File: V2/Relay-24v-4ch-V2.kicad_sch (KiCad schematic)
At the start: 25 parts, among them J1 DB141V-2.54-5P, J3 DB142V-5.08-2P, K1 SRD-24VDC-SL-A, K2 SRD-24VDC-SL-A, K3 SRD-24VDC-SL-A, K4 SRD-24VDC-SL-A

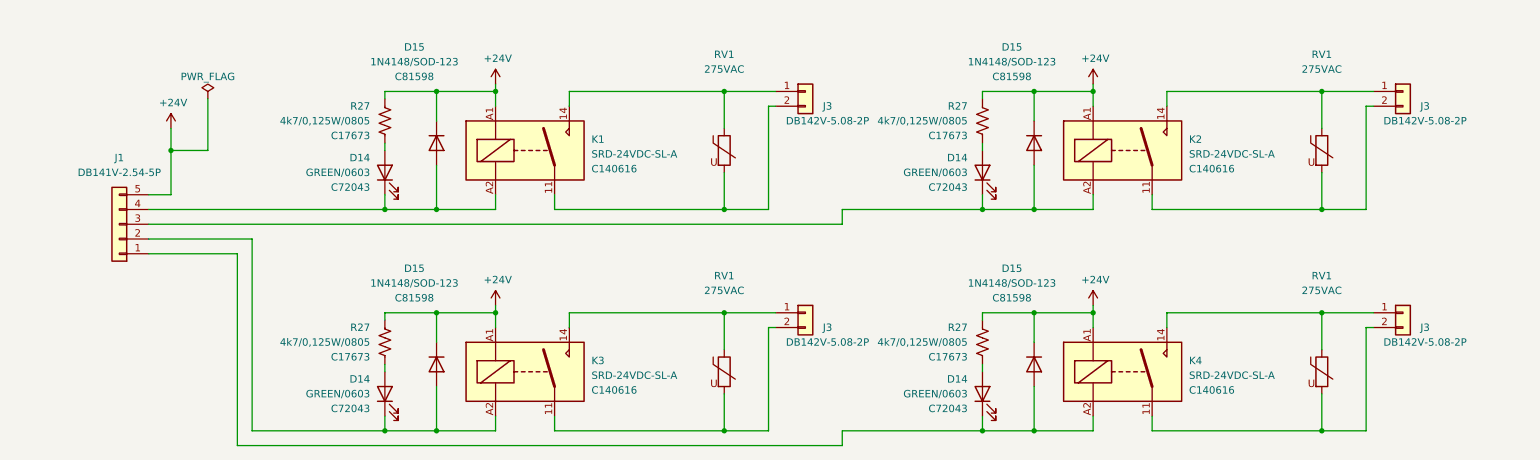
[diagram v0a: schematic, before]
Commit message: Redone everything
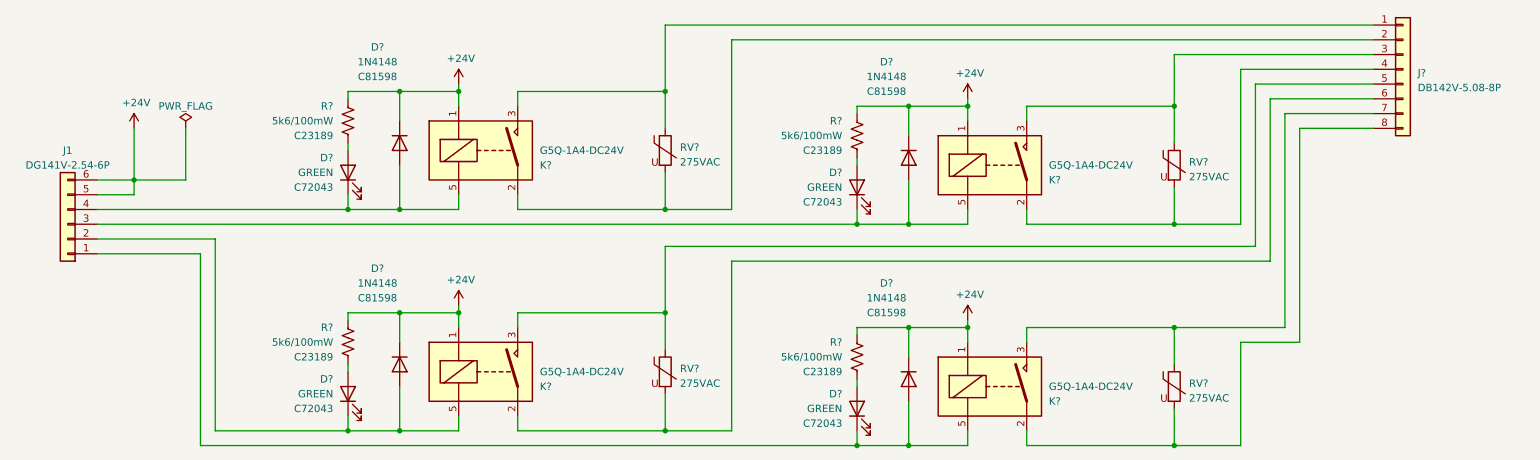
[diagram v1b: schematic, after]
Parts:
- removed J3 (x3): DB142V-5.08-2P, Tales:TerminalBlock_Dibo_DB142V-5.08-2P_1x02_P5.08mm_Vertical, symbol Connector_Generic:Conn_01x02
- removed K1, K2, K3, K4: SRD-24VDC-SL-A, Tales:Relay_SPST_Songle_SRD_FormA, symbol Tales:Songle_SRD
- added K? (x4): G5Q-1A4-DC24V, Tales:Relay_SPST_Omron-G5Q-1A, symbol Tales:G5Q-1A
- D? (x4): renamed from D14; value GREEN/0603 -> GREEN; Case 0603 -> (none); Package (none) -> 0603/1608
- D? (x4): renamed from D15; value 1N4148/SOD-123 -> 1N4148; Case SOD-123 -> (none); Package (none) -> SOD-123
- J1: value DB141V-2.54-5P -> DG141V-2.54-6P; footprint Tales:TerminalBlock_Dibo_DB141V-2.54-5P_1x05_P2.54mm_Vertical -> Tales:TerminalBlock_Dibo_DB141V-2.54-6P_1x06_P2.54mm_Vertical; symbol Connector_Generic:Conn_01x05 -> Connector_Generic:Conn_01x06; Mfr Dibo -> DIBO
- J?: renamed from J3; value DB142V-5.08-2P -> DB142V-5.08-8P; footprint Tales:TerminalBlock_Dibo_DB142V-5.08-2P_1x02_P5.08mm_Vertical -> Tales:TerminalBlock_Dibo_DB142V-5.08-8P_1x08_P5.08mm_Vertical; symbol Connector_Generic:Conn_01x02 -> Connector_Generic:Conn_01x08; LCSC Part # (none) -> C2898705; Mfr (none) -> DIBO; Mfr PN (none) -> DB142V-5.08-8P; Vendor PN (none) -> C2898705
- R? (x4): renamed from R27; value 4k7/0,125W/0805 -> 5k6/100mW; footprint Tales:R_0805_2012Metric -> Tales:R_0603_1608Metric; Case 0805/2012 -> (none); LCSC Part # C17673 -> C23189; Package (none) -> 0603/1608; Vendor PN C17673 -> C23189
- RV? (x4): renamed from RV1; JLCPCB BOM 0 -> 1; LCSC Part # (none) -> C2761646; Mfr Yageo -> Dersonic; Mfr PN 431KD10 -> RM07D431KC1IE100; Package (none) -> 9.5X5.08mm; Vendor Mouser -> JLCPCB; Vendor PN 603-431KD10 -> C2761646
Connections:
- net +24V: now also J1.6 (Pin_6), K?.1, K?.1, K?.1, K?.1
- net at D?.1 (K), D?.2 (A), J1.1 (Pin_1): now also K?.5
- net at D?.1 (K), D?.2 (A), J1.4 (Pin_4): now also K?.5
- net at D?.1 (K), D?.2 (A), J1.2 (Pin_2): now also K?.5
- net at D?.1 (K), D?.2 (A), J1.3 (Pin_3): now also K?.5
- net at RV?.1: now also J?.7 (Pin_7), K?.3
- net at RV?.2: now also J?.8 (Pin_8), K?.2
- net at RV?.1: now also J?.3 (Pin_3), K?.3
- net at RV?.2: now also J?.4 (Pin_4), K?.2
- net at J?.1 (Pin_1), RV?.1: now also K?.3
- net at J?.2 (Pin_2), RV?.2: now also K?.2
- net at RV?.1: now also J?.5 (Pin_5), K?.3
- net at RV?.2: now also J?.6 (Pin_6), K?.2
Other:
- moved on the sheet: D?, R?, RV?
